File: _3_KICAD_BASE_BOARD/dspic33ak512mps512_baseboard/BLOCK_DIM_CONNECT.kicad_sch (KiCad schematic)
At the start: 1 part, among them J1 HTEC8-160-01-X-DV-A-BL-X

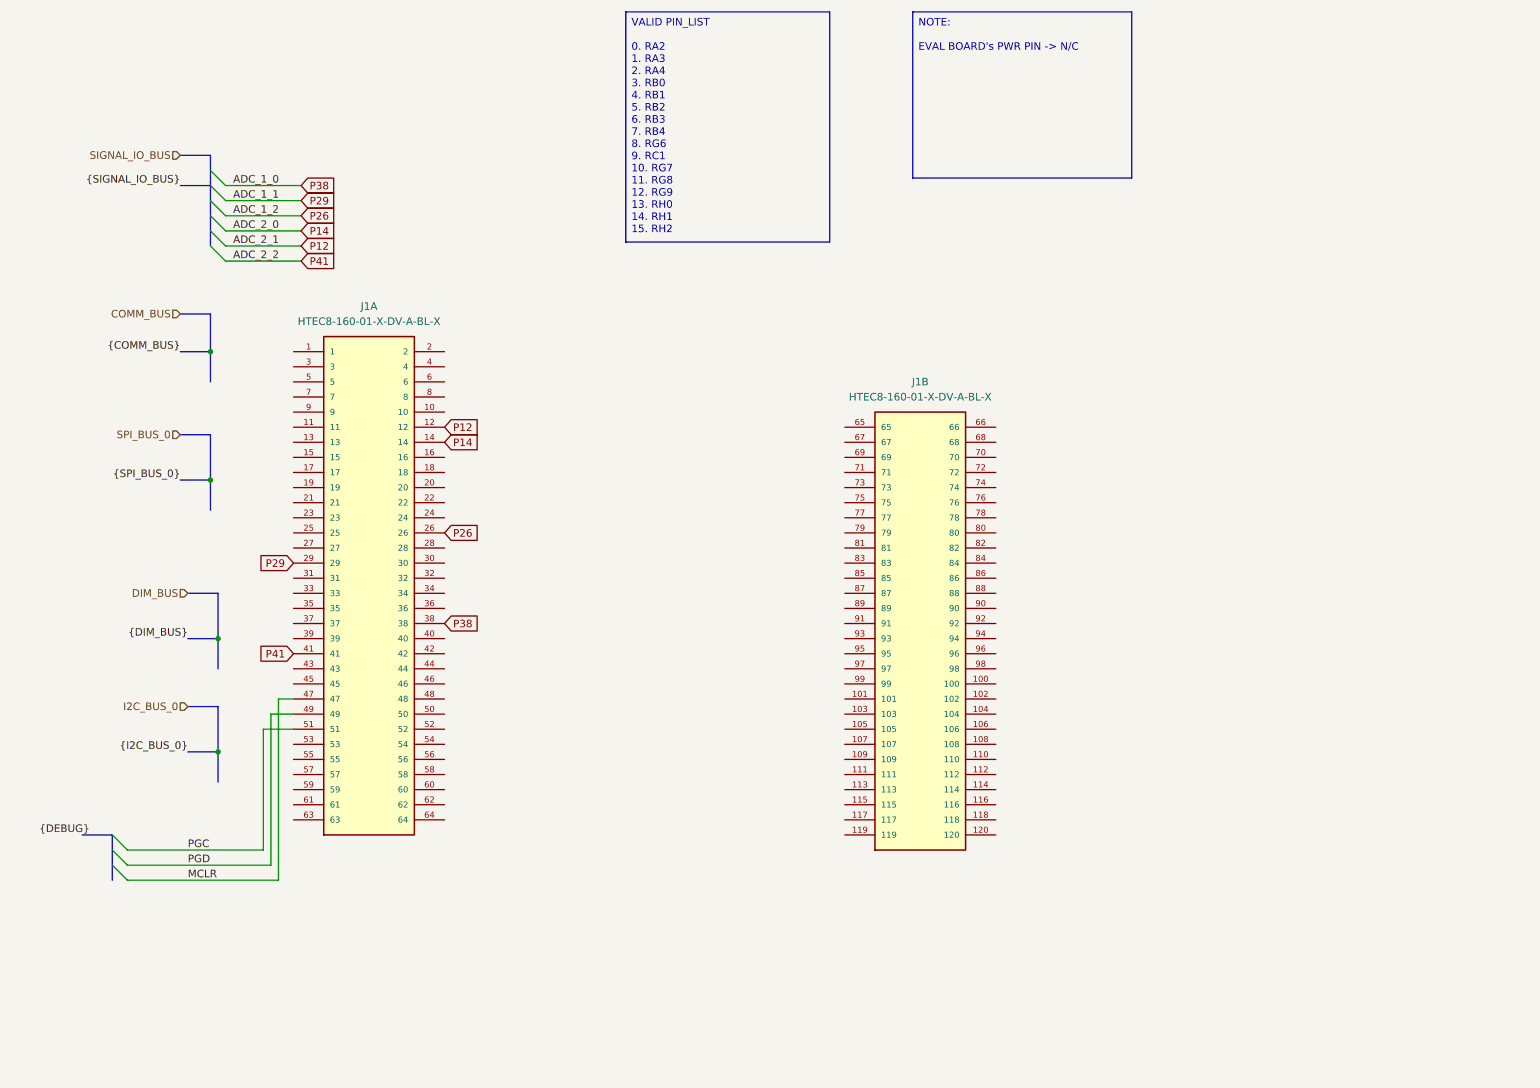
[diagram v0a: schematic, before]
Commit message: feat : 회로 작업중
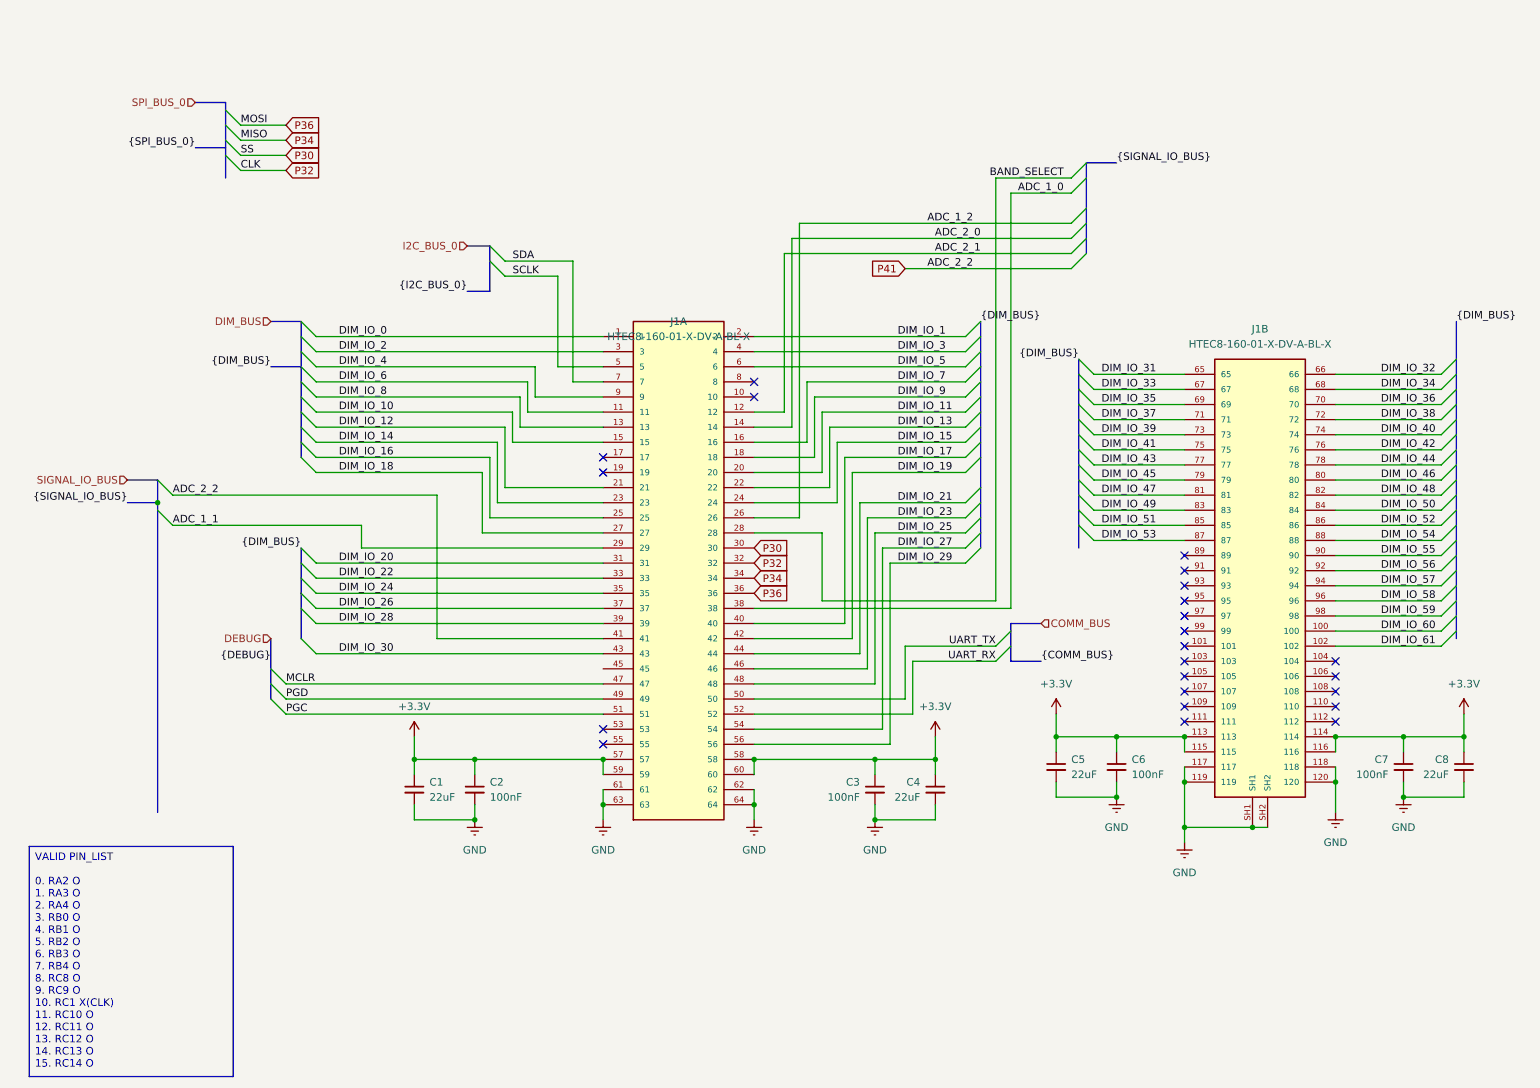
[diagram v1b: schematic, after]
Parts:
- added C1, C4, C5, C8: 22uF, Capacitor_SMD:C_0603_1608Metric, symbol Device:C_Small
- added C2, C3, C6, C7: 100nF, Capacitor_SMD:C_0603_1608Metric, symbol Device:C_Small
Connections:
- net DIM_IO_60: now reaches J1.100
- net DIM_IO_61: now reaches J1.102
- net +3.3V: now reaches J1.113
- net +3.3V: now also J1.114, J1.115, J1.116, J1.57, J1.58, J1.59, J1.60, C1.1, C2.1, C3.1, C4.1, C5.1, C6.1, C7.1, C8.1
- net GND: now reaches J1.117
- net GND: now also J1.118, J1.119, J1.120, J1.61, J1.62, J1.63, J1.64, J1.SH1, J1.SH2, C1.2, C2.2, C3.2, C4.2, C5.2, C6.2, C7.2, C8.2
- net DIM_IO_31: now reaches J1.65
- net DIM_IO_32: now reaches J1.66
- net DIM_IO_33: now reaches J1.67
- net DIM_IO_34: now reaches J1.68
- net DIM_IO_35: now reaches J1.69
- net DIM_IO_36: now reaches J1.70
- net DIM_IO_37: now reaches J1.71
- net DIM_IO_38: now reaches J1.72
- net DIM_IO_39: now reaches J1.73
- net DIM_IO_40: now reaches J1.74
- net DIM_IO_41: now reaches J1.75
- net DIM_IO_42: now reaches J1.76
- net DIM_IO_43: now reaches J1.77
- net DIM_IO_44: now reaches J1.78
- net DIM_IO_45: now reaches J1.79
- net DIM_IO_46: now reaches J1.80
- net DIM_IO_47: now reaches J1.81
- net DIM_IO_48: now reaches J1.82
- net DIM_IO_49: now reaches J1.83
- net DIM_IO_50: now reaches J1.84
- net DIM_IO_51: now reaches J1.85
- net DIM_IO_52: now reaches J1.86
- net DIM_IO_53: now reaches J1.87
- net DIM_IO_54: now reaches J1.88
- net DIM_IO_55: now reaches J1.90
- net DIM_IO_56: now reaches J1.92
- net DIM_IO_57: now reaches J1.94
- net DIM_IO_58: now reaches J1.96
- net DIM_IO_59: now reaches J1.98
- net DIM_IO_0: now reaches J1.1
- net DIM_IO_6: now reaches J1.11
- net DIM_IO_8: now reaches J1.13
- net DIM_IO_10: now reaches J1.15
- net DIM_IO_7: now reaches J1.16
- net DIM_IO_9: now reaches J1.18
- net DIM_IO_1: now reaches J1.2
- net DIM_IO_11: now reaches J1.20
- net DIM_IO_12: now reaches J1.21
- net DIM_IO_13: now reaches J1.22
- net DIM_IO_14: now reaches J1.23
- net DIM_IO_15: now reaches J1.24
- net DIM_IO_16: now reaches J1.25
- net DIM_IO_18: now reaches J1.27
- net BAND_SELECT: now reaches J1.28
- net DIM_IO_2: now reaches J1.3
- net P30: now reaches J1.30
- net DIM_IO_20: now reaches J1.31
- net P32: now reaches J1.32
- net DIM_IO_22: now reaches J1.33
- net P34: now reaches J1.34
- net DIM_IO_24: now reaches J1.35
- net P36: now reaches J1.36
- net DIM_IO_26: now reaches J1.37
- net DIM_IO_28: now reaches J1.39
- net DIM_IO_3: now reaches J1.4
- net DIM_IO_17: now reaches J1.40
- net DIM_IO_19: now reaches J1.42
- net DIM_IO_30: now reaches J1.43
- net DIM_IO_21: now reaches J1.44
- net DIM_IO_23: now reaches J1.46
- net DIM_IO_25: now reaches J1.48
- net SCLK: now reaches J1.5
- net UART_TX: now reaches J1.50
- net UART_RX: now reaches J1.52
- net DIM_IO_27: now reaches J1.54
- net DIM_IO_29: now reaches J1.56
- net DIM_IO_5: now reaches J1.6
- net SDA: now reaches J1.7
- net DIM_IO_4: now reaches J1.9
- net P12 renamed ADC_2_1
- net P14 renamed ADC_2_0
- net P26 renamed ADC_1_2
- net P29 renamed ADC_1_1
- net P38 renamed ADC_1_0
- no-connect marks 0 -> 23
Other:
- moved on the sheet: J1A
